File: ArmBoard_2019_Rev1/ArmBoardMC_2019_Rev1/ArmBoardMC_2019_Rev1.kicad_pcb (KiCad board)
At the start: 2 copper layers, 58 parts, among them U1 VNH5019A_E, U10 Limit_Switch7, U11 Limit_Switch2, U12 Limit_Switch4, U13 Limit_Switch6, U14 Limit_Switch8, U15 MAX_3232, U16 OKI, U17 Encoder_1, U18 Encoder_3, U19 Encoder_2, U2 VNH5019A_E, U20 Encoder_4, U3 TM4C129E_Launchpad, U5 VNH5019A_E, U6 VNH5019A_E, U7 Limit_Switch1, U8 Limit_Switch3, U9 Limit_Switch5

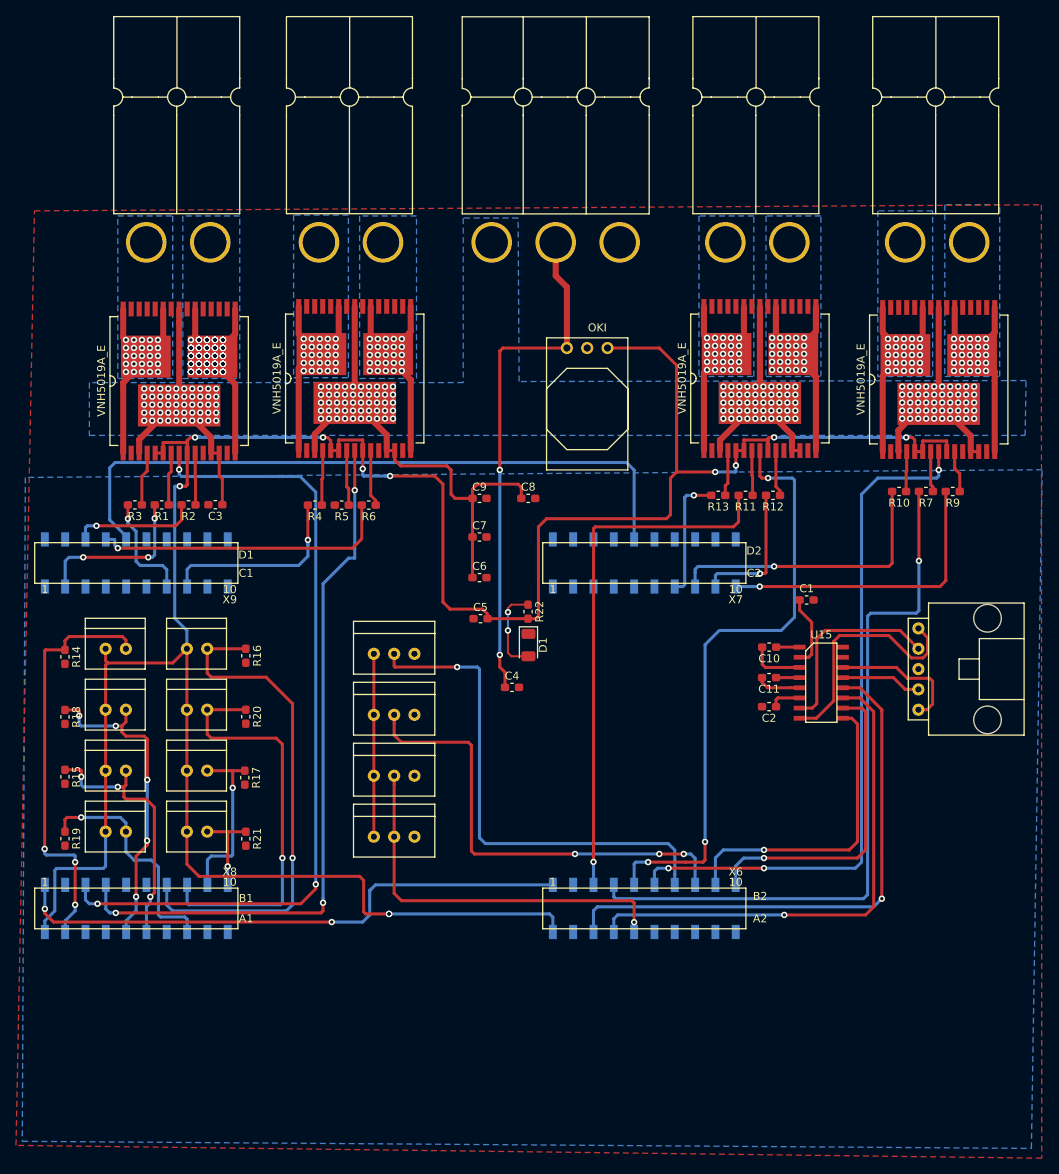
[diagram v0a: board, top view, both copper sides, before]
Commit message: Revert "Made some changes to board wiring"
This reverts commit da9662cbcf42a8357acbb6e05bfca608f18f2124.
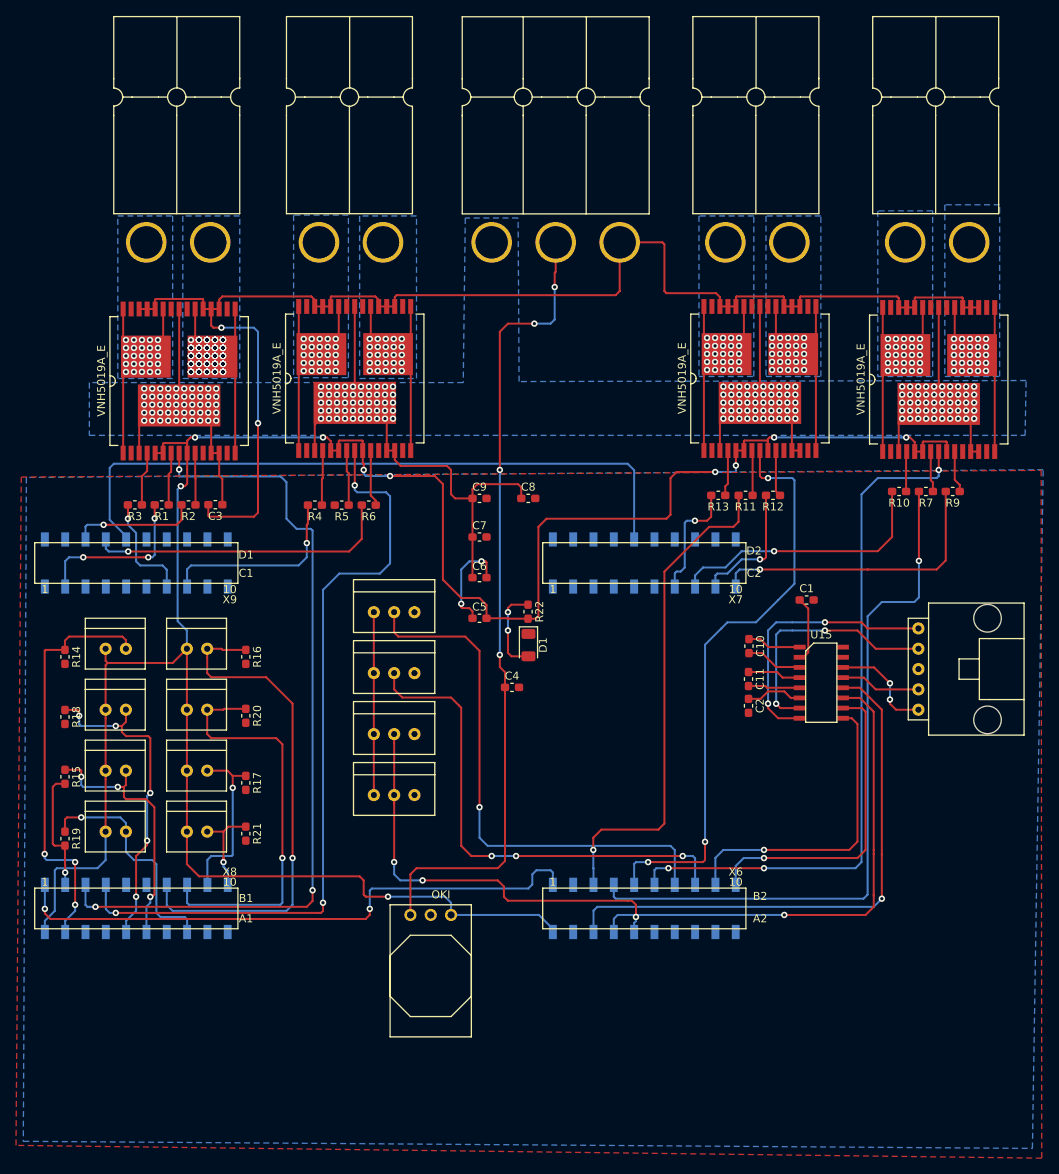
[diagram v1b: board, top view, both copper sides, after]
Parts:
- moved U16 73.5 mm to (84.3, 136.4)
- moved U17 5.21 mm to (79.8, 97.3)
- moved U20 5.21 mm to (79.8, 120.1)
- moved U18 5.21 mm to (79.8, 112.5)
- moved U19 5.21 mm to (79.8, 104.9)
- moved C11 2.57 mm to (129.1, 108.2), turned to 270 degrees
- moved C2 2.57 mm to (129.1, 111.5), turned to 270 degrees
- moved C10 2.53 mm to (129.2, 104.1), turned to 270 degrees
- moved R17 0.66 mm to (66.3, 121.2)
- moved R21 0.64 mm to (66.3, 127.5)
- moved R16 0.14 mm to (66.3, 105.4)
- moved C5 0.14 mm to (95.5, 100.6)
- moved R20 0.11 mm to (66.3, 112.8)
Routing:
- net GND: track 0.00 -> 201.2 mm, vias 0 -> 5
- net Logic_3.3V: track 355.1 -> 307.7 mm, vias 11 -> 10
- net /V+Log: track 64.6 -> 101.2 mm, vias 2 -> 4
- net I_Sense_2: track 129.3 -> 98.4 mm
- net RX_1_Tiva: track 92.7 -> 69.1 mm
- net Encoder3_PWM: track 64.3 -> 54.5 mm, vias 1 -> 3
- net TX_2_SL: track 24.6 -> 30.8 mm, vias 0 -> 2
- net LS_2: track 46.1 -> 41.2 mm
- net /Out_A1: track 25.1 -> 29.7 mm
- net /Out_B1: track 24.4 -> 28.8 mm
- net RX_2_SL: track 29.6 -> 33.7 mm, vias 0 -> 2
- net Net-(C11-Pad1): track 2.95 -> 6.95 mm
- net Encoder2_PWM: track 58.0 -> 61.8 mm
- net Net-(C10-Pad1): track 2.94 -> 6.76 mm
- net MOTOR3_PWM: track 66.5 -> 62.7 mm
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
